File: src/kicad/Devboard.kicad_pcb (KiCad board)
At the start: 4 copper layers, 47 x 35 mm, 49 parts, among them J1 USB_C_Receptacle_USB2.0_16P, J2 Conn_01x06, J3 Conn_01x06, J4 Conn_01x02, SW1 RESET, SW2 BOOT, U1 XC6220B331MR, U2 ESP32-C3, U3 W25Q128JVS, Y1 40MHz

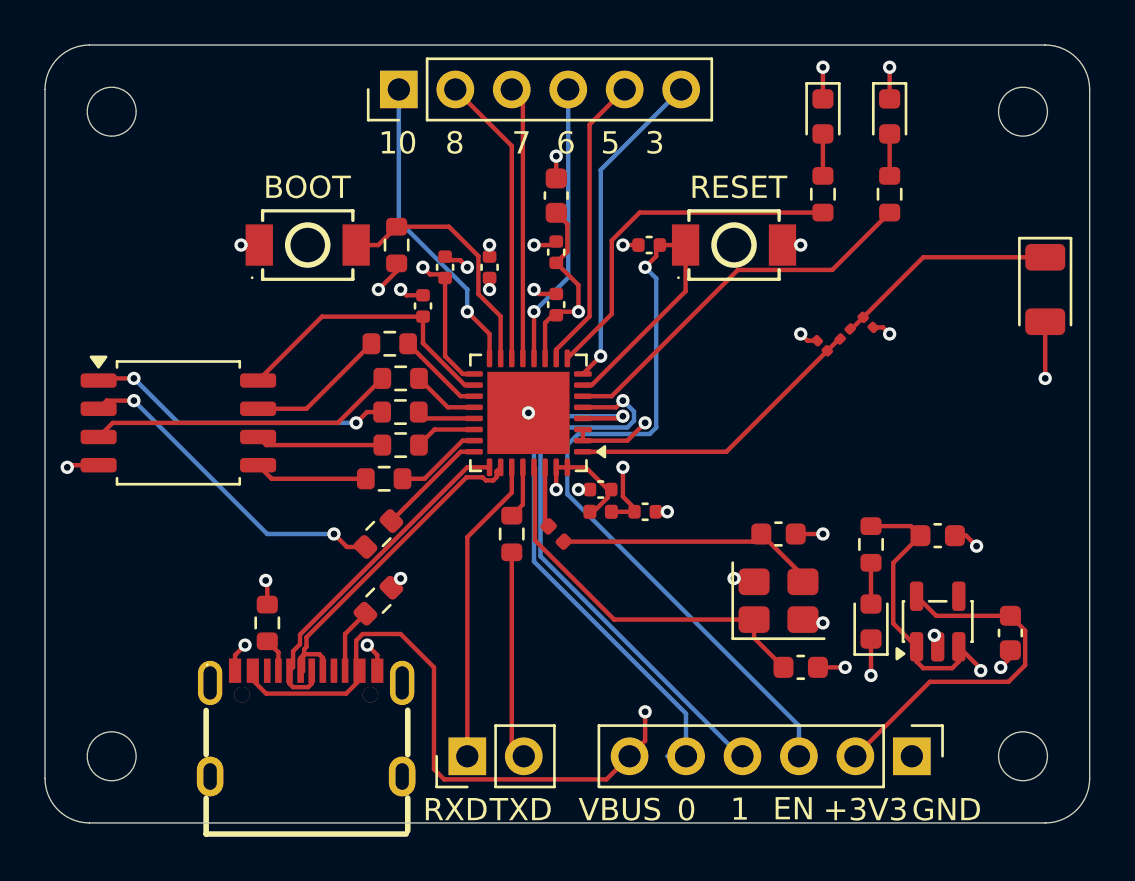
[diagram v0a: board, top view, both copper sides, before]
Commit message: Update project
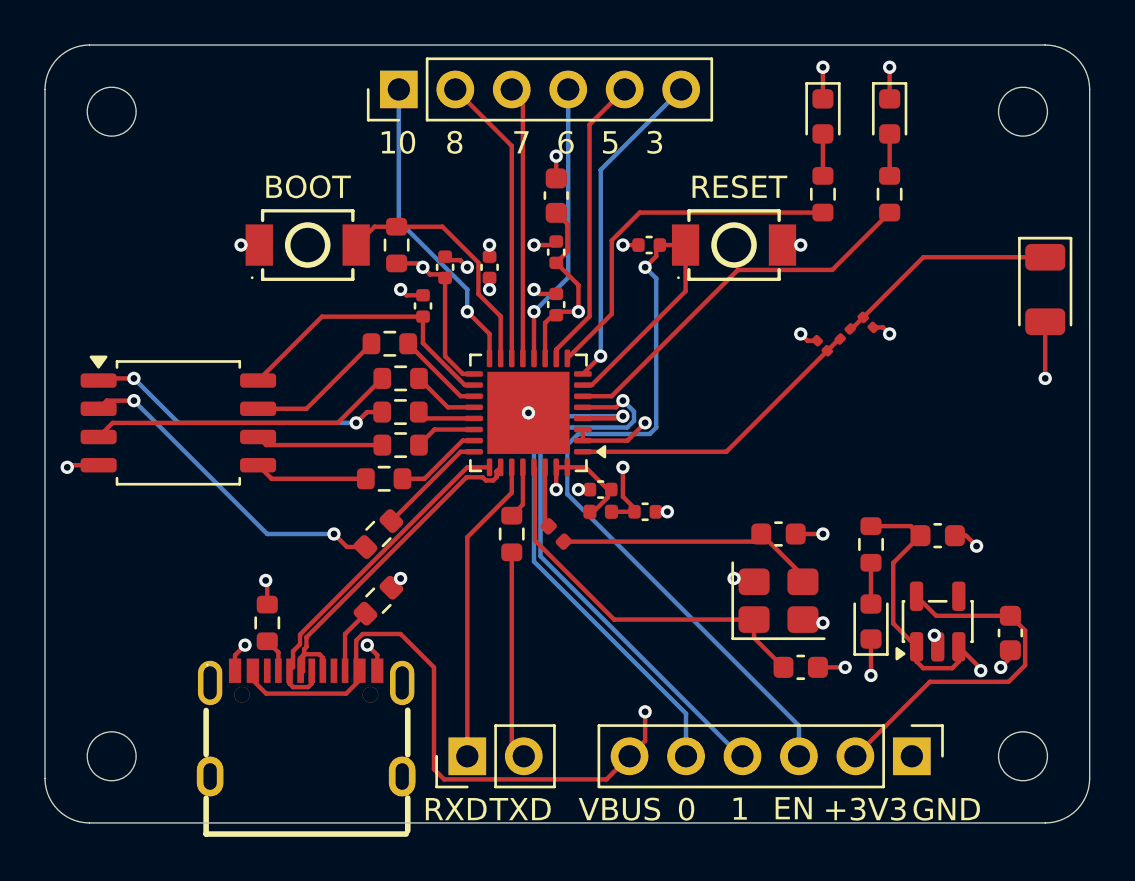
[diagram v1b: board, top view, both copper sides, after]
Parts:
- C11, C12: value 10uF -> 10pF
- turned R4 to 90 degrees
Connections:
- R4 pad 1: /GPIO9 -> +3.3V
- R4 pad 2: GND -> /GPIO9
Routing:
- net GND: track 33.2 -> 31.7 mm, vias 31 -> 30
- net +3.3V: track 38.5 -> 39.7 mm
- net /GPIO7: track 13.3 -> 12.3 mm
- net /GPIO0: track 24.1 -> 23.2 mm
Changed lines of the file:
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@@
 			)
 		)
-		(property "Value" "10uF"
+		(property "Value" "10pF"
 			(at 0 1.43 0)
 			(layer "F.Fab")
@@
 			)
 		)
-		(property "LCSC Part" "C96446"
+		(property "LCSC Part" "C1634"
 			(at 0 0 0)
 			(unlocked yes)
@@
 		(model "${EASYEDA2KICAD}/easyeda2kicad.3dshapes/USB-C-SMD_TYPE-C-6PIN-2MD-073.wrl"
 			(offset
-				(xyz 0 0 0)
+				(xyz 0 -1.5 1.5)
 			)
 			(scale
@@
 			)
 			(rotate
-				(xyz 0 0 0)
+				(xyz -0 -0 -0)
 			)
 		)
@@
 	(footprint "Resistor_SMD:R_0603_1608Metric"
 		(layer "F.Cu")
-		(at 155.82 87 -90)
+		(at 155.82 87 90)
 		(descr "Resistor SMD 0603 (1608 Metric), square (rectangular) end terminal, IPC-7351 nominal, (Body size source: IPC-SM-782 page 72, https://www.pcb-3d.com/wordpress/wp-content/uploads/ipc-sm-782a_amendment_1_and_2.pdf)")
 		(tags "resistor")
 		(property "Reference" "R4"
-			(at 0 -1.43 270)
+			(at 0 -1.43 90)
 			(layer "F.SilkS")
 			(hide yes)
@@
 		)
 		(property "Value" "10k"
-			(at 0 1.43 270)
+			(at 0 1.43 90)
 			(layer "F.Fab")
 			(effects
@@
 		)
 		(property "Datasheet" ""
-			(at 0 0 270)
+			(at 0 0 90)
 			(layer "F.Fab")
 			(hide yes)
@@
 		)
 		(property "Description" "Resistor"
-			(at 0 0 270)
+			(at 0 0 90)
 			(layer "F.Fab")
 			(hide yes)
@@
 		)
 		(property "KiLib_Generator" "SMD_2terminal_chip_molded"
-			(at 0 0 270)
+			(at 0 0 90)
 			(layer "F.SilkS")
 			(hide yes)
@@
 		)
 		(property "LCSC Part" "C2930027"
-			(at 0 0 270)
+			(at 0 0 90)
 			(unlocked yes)
 			(layer "F.Fab")
@@
 		)
 		(property "KLC_S3.3" ""
-			(at 0 0 270)
+			(at 0 0 90)
 			(unlocked yes)
 			(layer "F.Fab")
@@
 		)
 		(property "KLC_S4.1" ""
-			(at 0 0 270)
+			(at 0 0 90)
 			(unlocked yes)
 			(layer "F.Fab")
@@
 		(duplicate_pad_numbers_are_jumpers no)
 		(fp_line
-			(start -0.237258 0.5225)
-			(end 0.237258 0.5225)
+			(start -0.237258 -0.5225)
+			(end 0.237258 -0.5225)
 			(stroke
 				(width 0.12)
@@
 		)
 		(fp_line
-			(start -0.237258 -0.5225)
-			(end 0.237258 -0.5225)
+			(start -0.237258 0.5225)
+			(end 0.237258 0.5225)
 			(stroke
 				(width 0.12)
@@
 		)
 		(fp_text user "${REFERENCE}"
-			(at 0 0 270)
+			(at 0 0 90)
 			(layer "F.Fab")
 			(effects
@@
 		)
 		(pad "1" smd roundrect
-			(at -0.825 0 270)
+			(at -0.825 0 90)
 			(size 0.8 0.95)
 			(layers "F.Cu" "F.Mask" "F.Paste")
 			(roundrect_rratio 0.25)
-			(net "/GPIO9")
+			(net "+3.3V")
 			(pintype "passive")
 		)
 		(pad "2" smd roundrect
-			(at 0.825 0 270)
+			(at 0.825 0 90)
 			(size 0.8 0.95)
 			(layers "F.Cu" "F.Mask" "F.Paste")
 			(roundrect_rratio 0.25)
-			(net "GND")
+			(net "/GPIO9")
 			(pintype "passive")
 		)
@@
 			)
 		)
-		(property "Value" "10uF"
+		(property "Value" "10pF"
 			(at 0 1.43 0)
 			(layer "F.Fab")
@@
 			)
 		)
-		(property "LCSC Part" "C96446"
+		(property "LCSC Part" "C1634"
 			(at 0 0 0)
 			(unlocked yes)
@@
 			)
 		)
-		(property "LCSC Part" "C23733"
+		(property "LCSC Part" "C69335"
 			(at 0 0 270)
 			(unlocked yes)
@@
 	)
 	(segment
-		(start 155.82 87.825)
-		(end 155.82 88.18)
-		(width 0.2)
-		(layer "F.Cu")
-		(net "GND")
-	)
-	(segment
 		(start 177.1625 104.725)
 		(end 177.1625 106.3625)
@@
 	)
 	(segment
-		(start 155.82 88.18)
-		(end 155 89)
-		(width 0.2)
-		(layer "F.Cu")
-		(net "GND")
-	)
-	(segment
 		(start 158 87.68)
 		(end 158.68 87.68)
@@
 	)
 	(via
-		(at 155 89)
-		(size 0.6)
-		(drill 0.3)
-		(layers "F.Cu" "B.Cu")
-		(net "GND")
-	)
-	(via
 		(at 160 87)
 		(size 0.6)
@@
 	)
 	(segment
+		(start 155.82 87.825)
+		(end 156.825 87.825)
+		(width 0.2)
+		(layer "F.Cu")
+		(net "+3.3V")
+	)
+	(segment
 		(start 163.93 90.07)
 		(end 164 90)
@@
 	)
 	(segment
+		(start 156.825 87.825)
+		(end 157 88)
+		(width 0.2)
+		(layer "F.Cu")
+		(net "+3.3V")
+	)
+	(segment
 		(start 158 92)
 		(end 158 88.32)
@@
 	)
 	(segment
-		(start 168 110)
-		(end 168.84 110)
-		(width 0.2)
-		(layer "B.Cu")
-		(net "/GPIO0")
-	)
-	(segment
 		(start 168.84 108.082893)
 		(end 168.84 110)
@@
 	)
 	(segment
-		(start 161.5 80.5)
-		(end 161 80)
+		(start 161 80)
+		(end 161.5 80.5)
 		(width 0.2)
 		(layer "F.Cu")
@@
 	)
 	(segment
-		(start 161.5 92.1)
-		(end 161.5 79.5)
+		(start 161.5 80.5)
+		(end 161.5 92.1)
 		(width 0.2)
 		(layer "F.Cu")
@@
 	)
 	(segment
-		(start 159.5 89.207107)
-		(end 159.5 87.5)
+		(start 160.5 92.1)
+		(end 160.5 90.207107)
 		(width 0.2)
 		(layer "F.Cu")
@@
 	)
 	(segment
-		(start 159.5 87.5)
-		(end 158.175 86.175)
+		(start 154.825 86.175)
+		(end 154 87)
 		(width 0.2)
 		(layer "F.Cu")
@@
 	)
 	(segment
-		(start 154 87)
-		(end 154.995 87)
+		(start 159.5 89.207107)
+		(end 159.5 87.792893)
 		(width 0.2)
 		(layer "F.Cu")
@@
 	)
 	(segment
-		(start 160.5 90.207107)
-		(end 159.5 89.207107)
+		(start 157.882107 86.175)
+		(end 155.82 86.175)
 		(width 0.2)
 		(layer "F.Cu")
@@
 	)
 	(segment
-		(start 154.995 87)
-		(end 155.82 86.175)
+		(start 155.82 86.175)
+		(end 154.825 86.175)
 		(width 0.2)
 		(layer "F.Cu")
@@
 	)
 	(segment
-		(start 160.5 92.1)
-		(end 160.5 90.207107)
+		(start 159.5 87.792893)
+		(end 157.882107 86.175)
 		(width 0.2)
 		(layer "F.Cu")
@@
 	)
 	(segment
-		(start 158.175 86.175)
-		(end 155.82 86.175)
+		(start 160.5 90.207107)
+		(end 159.5 89.207107)
 		(width 0.2)
 		(layer "F.Cu")
@@
 	)
 	(segment
-		(start 154.15 106.15)
-		(end 154.15 106.58)
-		(width 0.2)
-		(layer "F.Cu")
-		(net "VBUS")
-	)
-	(segment
 		(start 166.3 110)
 		(end 167 109.3)
@@
 	)
 	(segment
-		(start 149.95 107.18)
-		(end 149.35 106.58)
-		(width 0.2)
-		(layer "F.Cu")
-		(net "VBUS")
-	)
-	(segment
 		(start 179.512501 106.0375)
 		(end 179.2125 105.737499)
@@
 	)
 	(segment
-		(start 181.1125 105.075)
-		(end 181.1625 105.075)
+		(start 149.95 107.18)
+		(end 149.35 106.58)
 		(width 0.2)
 		(layer "F.Cu")
@@
 	)
 	(segment
-		(start 153.55 107.18)
-		(end 149.95 107.18)
+		(start 181.1125 105.075)
+		(end 181.1625 105.075)
 		(width 0.2)
 		(layer "F.Cu")
@@
 	)
 	(segment
-		(start 149.35 106.58)
-		(end 149.35 106.15)
-		(width 0.2)
-		(layer "F.Cu")
-		(net "VBUS")
-	)
-	(segment
 		(start 178.1625 101.3)
 		(end 179.3875 100.075)
@@
 	)
 	(segment
+		(start 153.55 107.18)
+		(end 149.95 107.18)
+		(width 0.2)
+		(layer "F.Cu")
+		(net "VBUS")
+	)
+	(segment
+		(start 149.35 106.58)
+		(end 149.35 106.15)
+		(width 0.2)
+		(layer "F.Cu")
+		(net "VBUS")
+	)
+	(segment
 		(start 165.26 111.04)
 		(end 166.3 110)
@@
 	)
 	(segment
+		(start 154.15 106.58)
+		(end 153.55 107.18)
+		(width 0.2)
+		(layer "F.Cu")
+		(net "VBUS")
+	)
+	(segment
 		(start 178.1625 104.025)
 		(end 178.1625 101.3)
@@
 	)
 	(segment
-		(start 154.15 106.58)
-		(end 153.55 107.18)
+		(start 154.15 106.15)
+		(end 154.15 106.58)
 		(width 0.2)
 		(layer "F.Cu")
